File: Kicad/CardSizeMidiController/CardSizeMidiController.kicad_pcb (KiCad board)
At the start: 2 copper layers, 85.7 x 54 mm, 41 parts, among them J1 USB_B, J2 Conn_02x03_Odd_Even, J3 MIDI OUT, J4 AudioJack3, J5 Screw_Terminal_01x01, J6 Screw_Terminal_01x01, J7 Screw_Terminal_01x01, J8 Screw_Terminal_01x01, SW0 SW_Push, SW1 SW_Push, SW2 SW_Push, SW3 SW_Push, SW4 SW_Push, SW5 SW_Push, U1 ATmega328P-AU, Y1 16MHz

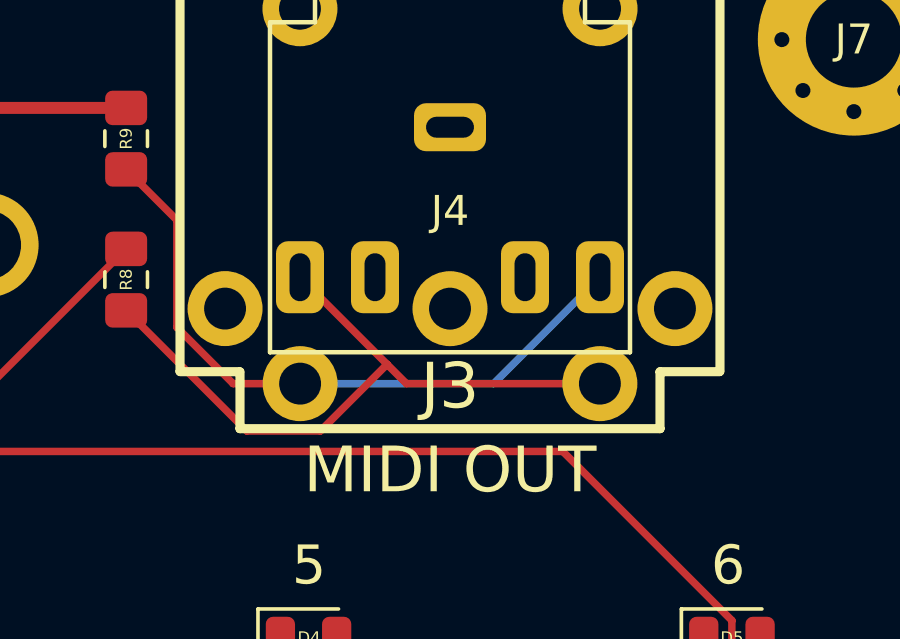
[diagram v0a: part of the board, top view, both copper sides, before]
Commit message: small layout changes
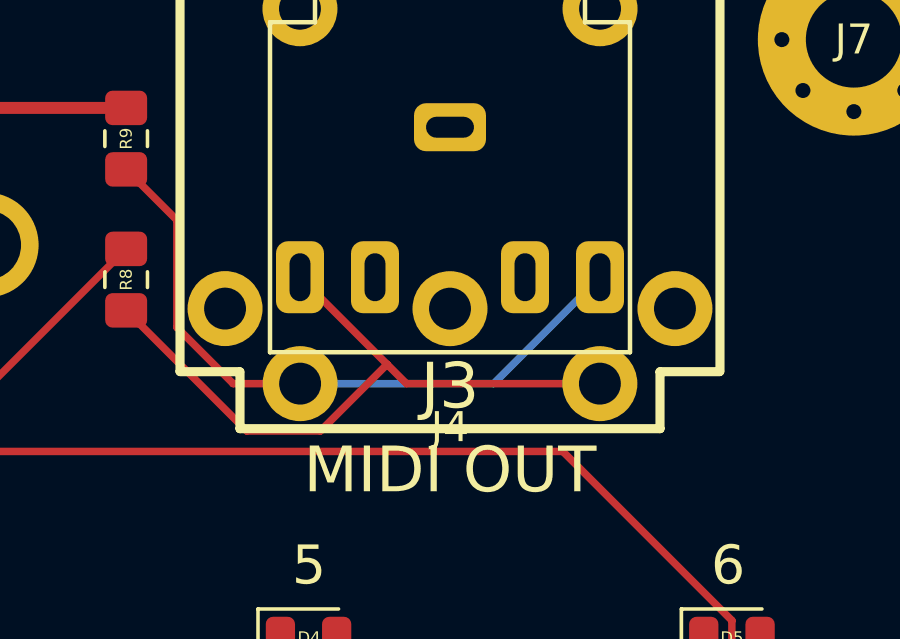
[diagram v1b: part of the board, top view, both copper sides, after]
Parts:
- J4: footprint SensaiLib:Jack stereo tayda -> SensaiLib:Jack stereo tayda no extra holes
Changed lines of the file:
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@@
     (add_net GND)
+  )
+  (module "SensaiLib:Jack stereo tayda no extra holes" (layer F.Cu)
+    (at 68.707 6.477 180)
+    (fp_text reference J4 (at 0 -10 180) (layer F.SilkS)
+      (effects (font (size 1 1) (thickness 0.15)))
+    )
+    (fp_text value AudioJack3 (at 0 -8.5 180) (layer F.Fab)
+      (effects (font (size 1 1) (thickness 0.15)))
+    )
+    (fp_line (start -4.5 3.5) (end -4.5 4.5) (layer F.SilkS) (width 0.15))
+    (fp_line (start 3 4.5) (end 3 6.5) (layer F.SilkS) (width 0.15))
+    (fp_line (start 6 3.5) (end 4.5 3.5) (layer F.SilkS) (width 0.15))
+    (fp_line (start -4.5 3.5) (end -6 3.5) (layer F.SilkS) (width 0.15))
+    (fp_line (start 4.5 4.5) (end -4.5 4.5) (layer F.SilkS) (width 0.15))
+    (fp_line (start 6 -7.5) (end 6 3.5) (layer F.SilkS) (width 0.15))
+    (fp_line (start -2.95 4.5) (end -2.95 6.5) (layer F.SilkS) (width 0.15))
+    (fp_line (start 4.5 3.5) (end 4.5 4.5) (layer F.SilkS) (width 0.15))
+    (fp_line (start 3 6.5) (end -2.95 6.5) (layer F.SilkS) (width 0.15))
+    (fp_line (start -2.9 5.5) (end 3 5.5) (layer F.SilkS) (width 0.15))
+    (fp_line (start -6 3.5) (end -6 -7.5) (layer F.SilkS) (width 0.15))
+    (fp_line (start -6 -7.5) (end 6 -7.5) (layer F.SilkS) (width 0.15))
+    (pad S thru_hole roundrect (at 0 0 180) (size 2.4 1.6) (drill oval 1.6 0.7) (layers *.Cu *.Mask) (roundrect_rratio 0.25)
+      (net 1 GND))
+    (pad TN thru_hole roundrect (at 2.5 -5 180) (size 1.6 2.4) (drill oval 0.7 1.6) (layers *.Cu *.Mask) (roundrect_rratio 0.25))
+    (pad RN thru_hole roundrect (at -2.5 -5 180) (size 1.6 2.4) (drill oval 0.7 1.6) (layers *.Cu *.Mask) (roundrect_rratio 0.25))
+    (pad T thru_hole roundrect (at 5 -5 180) (size 1.6 2.4) (drill oval 0.7 1.6) (layers *.Cu *.Mask) (roundrect_rratio 0.25)
+      (net 38 "Net-(J3-Pad5)"))
+    (pad R thru_hole roundrect (at -5 -5 180) (size 1.6 2.4) (drill oval 0.7 1.6) (layers *.Cu *.Mask) (roundrect_rratio 0.25)
+      (net 36 "Net-(J3-Pad4)"))
   )
   (module Button_Switch_THT:SW_PUSH_6mm_H5mm (layer F.Cu)
@@
     )
   )
-  (module "SensaiLib:Jack stereo tayda" (layer F.Cu)
-    (at 68.707 6.477 180)
-    (fp_text reference J4 (at 0 -2.794 180) (layer F.SilkS)
-      (effects (font (size 1 1) (thickness 0.15)))
-    )
-    (fp_text value AudioJack3 (at -0.2 -10.8 180) (layer F.Fab)
-      (effects (font (size 1 1) (thickness 0.15)))
-    )
-    (fp_line (start -6 -7.5) (end 6 -7.5) (layer F.SilkS) (width 0.15))
-    (fp_line (start 6 -7.5) (end 6 3.5) (layer F.SilkS) (width 0.15))
-    (fp_line (start 4.5 4.5) (end -4.5 4.5) (layer F.SilkS) (width 0.15))
-    (fp_line (start -6 3.5) (end -6 -7.5) (layer F.SilkS) (width 0.15))
-    (fp_line (start 3 4.5) (end 3 6.5) (layer F.SilkS) (width 0.15))
-    (fp_line (start 3 6.5) (end -2.95 6.5) (layer F.SilkS) (width 0.15))
-    (fp_line (start -2.95 4.5) (end -2.95 6.5) (layer F.SilkS) (width 0.15))
-    (fp_line (start -4.5 3.5) (end -4.5 4.5) (layer F.SilkS) (width 0.15))
-    (fp_line (start 4.5 3.5) (end 4.5 4.5) (layer F.SilkS) (width 0.15))
-    (fp_line (start -4.5 3.5) (end -6 3.5) (layer F.SilkS) (width 0.15))
-    (fp_line (start 6 3.5) (end 4.5 3.5) (layer F.SilkS) (width 0.15))
-    (fp_line (start -2.9 5.5) (end 3 5.5) (layer F.SilkS) (width 0.15))
-    (pad R thru_hole roundrect (at -5 -5 180) (size 1.6 2.4) (drill oval 0.7 1.6) (layers *.Cu *.Mask) (roundrect_rratio 0.25)
-      (net 36 "Net-(J3-Pad4)"))
-    (pad T thru_hole roundrect (at 5 -5 180) (size 1.6 2.4) (drill oval 0.7 1.6) (layers *.Cu *.Mask) (roundrect_rratio 0.25)
-      (net 38 "Net-(J3-Pad5)"))
-    (pad RN thru_hole roundrect (at -2.5 -5 180) (size 1.6 2.4) (drill oval 0.7 1.6) (layers *.Cu *.Mask) (roundrect_rratio 0.25))
-    (pad TN thru_hole roundrect (at 2.5 -5 180) (size 1.6 2.4) (drill oval 0.7 1.6) (layers *.Cu *.Mask) (roundrect_rratio 0.25))
-    (pad S thru_hole roundrect (at 0 0 180) (size 2.4 1.6) (drill oval 1.6 0.7) (layers *.Cu *.Mask) (roundrect_rratio 0.25)
-      (net 1 GND))
-  )
   (module SensaiLib:din-5 (layer F.Cu)
